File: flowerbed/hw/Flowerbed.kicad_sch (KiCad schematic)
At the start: 24 parts, among them J1 Conn_01x04, J2 Conn_01x04, U2 STM32G030F6Px, U2 VL53L0X, U3 W25Q16JVSS, U4 MAX98357AETE+, X1 12.288MHz

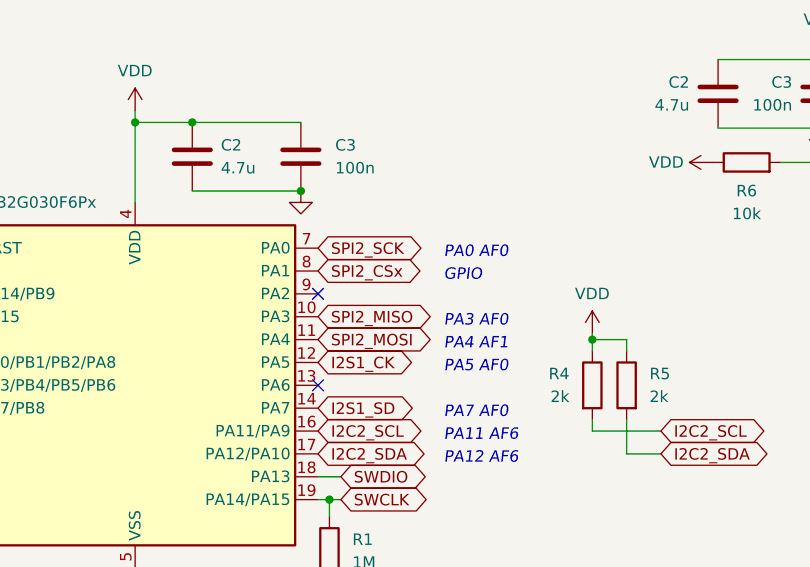
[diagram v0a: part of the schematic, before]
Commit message: Route flowerbed unit (!)
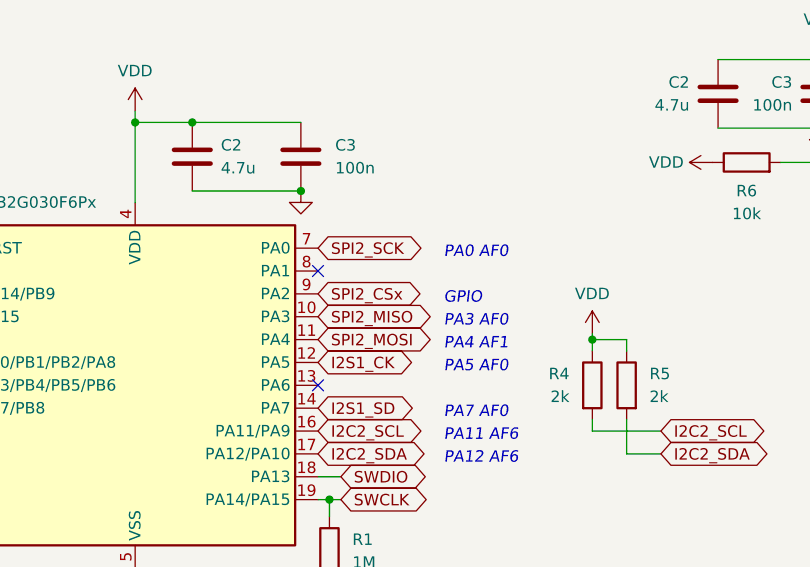
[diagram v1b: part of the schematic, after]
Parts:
- C2, C3: footprint Capacitor_SMD:C_0603_1608Metric -> Capacitor_SMD:C_0402_1005Metric
- U4: footprint Package_DFN_QFN:QFN-16-1EP_3x3mm_P0.5mm_EP1.45x1.45mm -> Flowerbed_footprints:QFN-16_3x3mm_P0.5mm
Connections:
- net SPI2_CSx: now also U2.9 (PA2); no longer U2.8 (PA1)
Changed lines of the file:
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@@
   (junction (at 147.32 47.625) (diameter 0) (color 0 0 0 0)
   )
-  (no_connect (at 149.225 59.055))
   (no_connect (at 238.125 123.19))
   (no_connect (at 108.585 53.975))
@@
   (no_connect (at 246.38 35.56))
   (no_connect (at 149.225 69.215))
+  (no_connect (at 149.225 56.515))
   (no_connect (at 191.135 125.73))
   (no_connect (at 212.725 148.59))
@@
     (effects (font (size 1.27 1.27) italic) (justify left bottom))
   )
-  (text "GPIO" (at 163.195 57.785 0)
-    (effects (font (size 1.27 1.27) italic) (justify left bottom))
-  )
   (text "PA3 AF0" (at 163.195 62.865 0)
     (effects (font (size 1.27 1.27) italic) (justify left bottom))
@@
   )
   (text "PA0 AF0" (at 163.195 55.245 0)
+    (effects (font (size 1.27 1.27) italic) (justify left bottom))
+  )
+  (text "GPIO" (at 163.195 60.325 0)
     (effects (font (size 1.27 1.27) italic) (justify left bottom))
   )
@@
     )
   )
+  (global_label "SPI2_CSx" (shape bidirectional) (at 149.225 59.055 0) (fields_autoplaced)
+    (effects (font (size 1.27 1.27)) (justify left))
+    (property "Intersheetrefs" "${INTERSHEET_REFS}" (at 162.0905 59.055 0)
+      (effects (font (size 1.27 1.27)) (justify left) hide)
+    )
+  )
   (global_label "SPI2_MISO" (shape bidirectional) (at 229.235 78.105 180) (fields_autoplaced)
     (effects (font (size 1.27 1.27)) (justify right))
@@
     )
   )
-  (global_label "SPI2_CSx" (shape bidirectional) (at 149.225 56.515 0) (fields_autoplaced)
-    (effects (font (size 1.27 1.27)) (justify left))
-    (property "Intersheetrefs" "${INTERSHEET_REFS}" (at 162.0905 56.515 0)
-      (effects (font (size 1.27 1.27)) (justify left) hide)
-    )
-  )
   (global_label "I2S1_CK" (shape bidirectional) (at 149.225 66.675 0) (fields_autoplaced)
     (effects (font (size 1.27 1.27)) (justify left))
@@
       (effects (font (size 1.27 1.27)))
     )
-    (property "Footprint" "Package_DFN_QFN:QFN-16-1EP_3x3mm_P0.5mm_EP1.45x1.45mm" (at 234.315 110.49 0)
+    (property "Footprint" "Flowerbed_footprints:QFN-16_3x3mm_P0.5mm" (at 234.315 110.49 0)
       (effects (font (size 1.27 1.27)) (justify left) hide)
     )
@@
       (effects (font (size 1.27 1.27)) (justify left))
     )
-    (property "Footprint" "Capacitor_SMD:C_0603_1608Metric" (at 192.7098 40.64 0)
+    (property "Footprint" "Capacitor_SMD:C_0402_1005Metric" (at 192.7098 40.64 0)
       (effects (font (size 1.27 1.27)) hide)
     )
@@
       (effects (font (size 1.27 1.27)) (justify left))
     )
-    (property "Footprint" "Capacitor_SMD:C_0603_1608Metric" (at 204.1398 40.64 0)
-      (effects (font (size 1.27 1.27)) hide)
-    )
+    (property "Footprint" "Capacitor_SMD:C_0402_1005Metric" (at 204.1398 40.64 0)
+      (effects (font (size 1.27 1.27)) hide)
+    )
